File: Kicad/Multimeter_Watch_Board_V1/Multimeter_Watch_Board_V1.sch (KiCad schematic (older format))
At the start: 38 parts, among them J1 AudioJack3_Ground_renamedPins, J2 AudioJack3_Ground_renamedPins, J3 AudioJack3_Ground_renamedPins, J4 Conn_01x16_Female, J5 Conn_01x16_Female, U1 PCF85163-SO08, U2 AD8592, Y1 32kHz

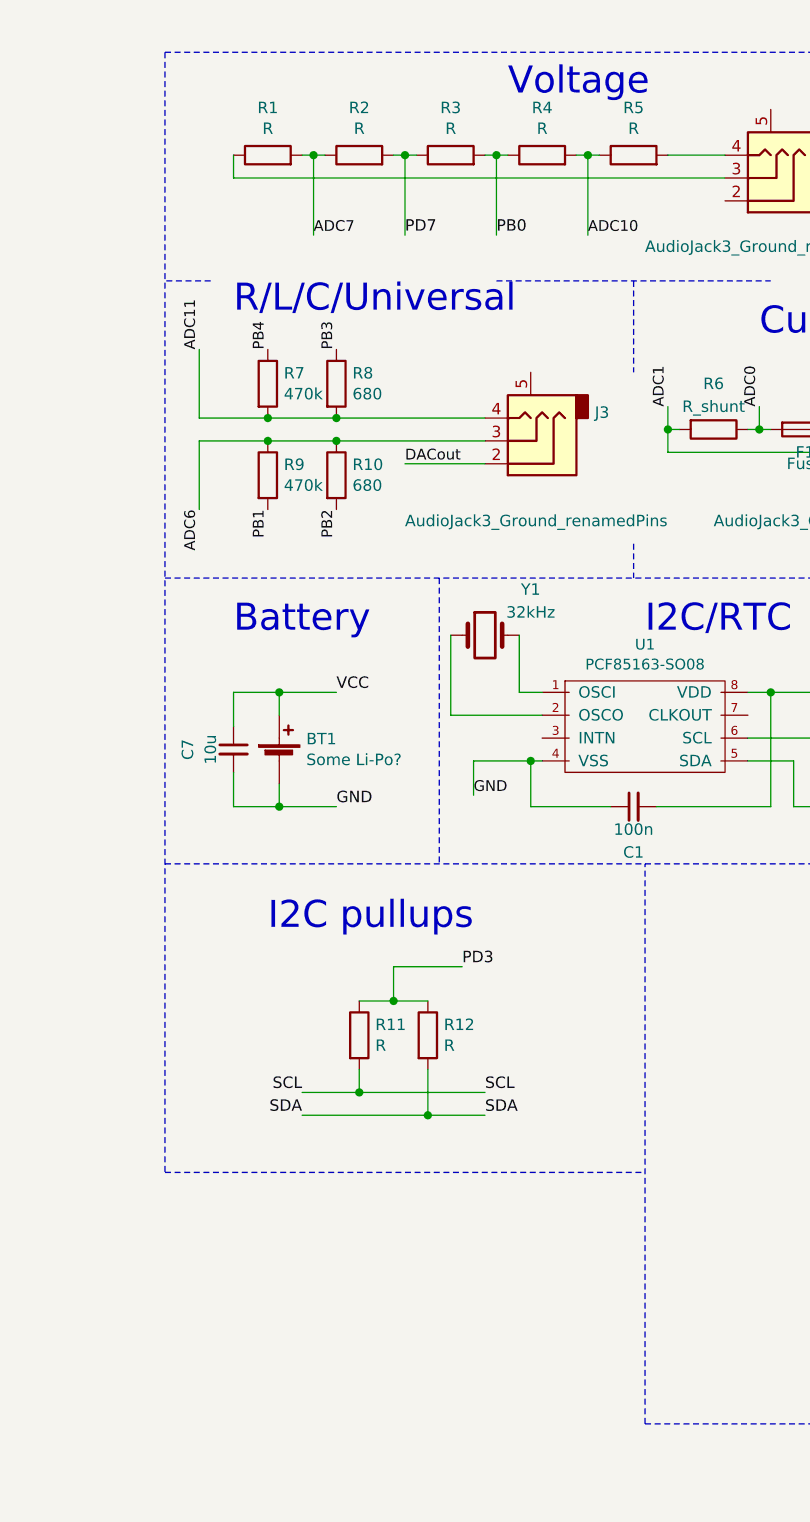
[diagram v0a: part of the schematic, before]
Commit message: reset pullup
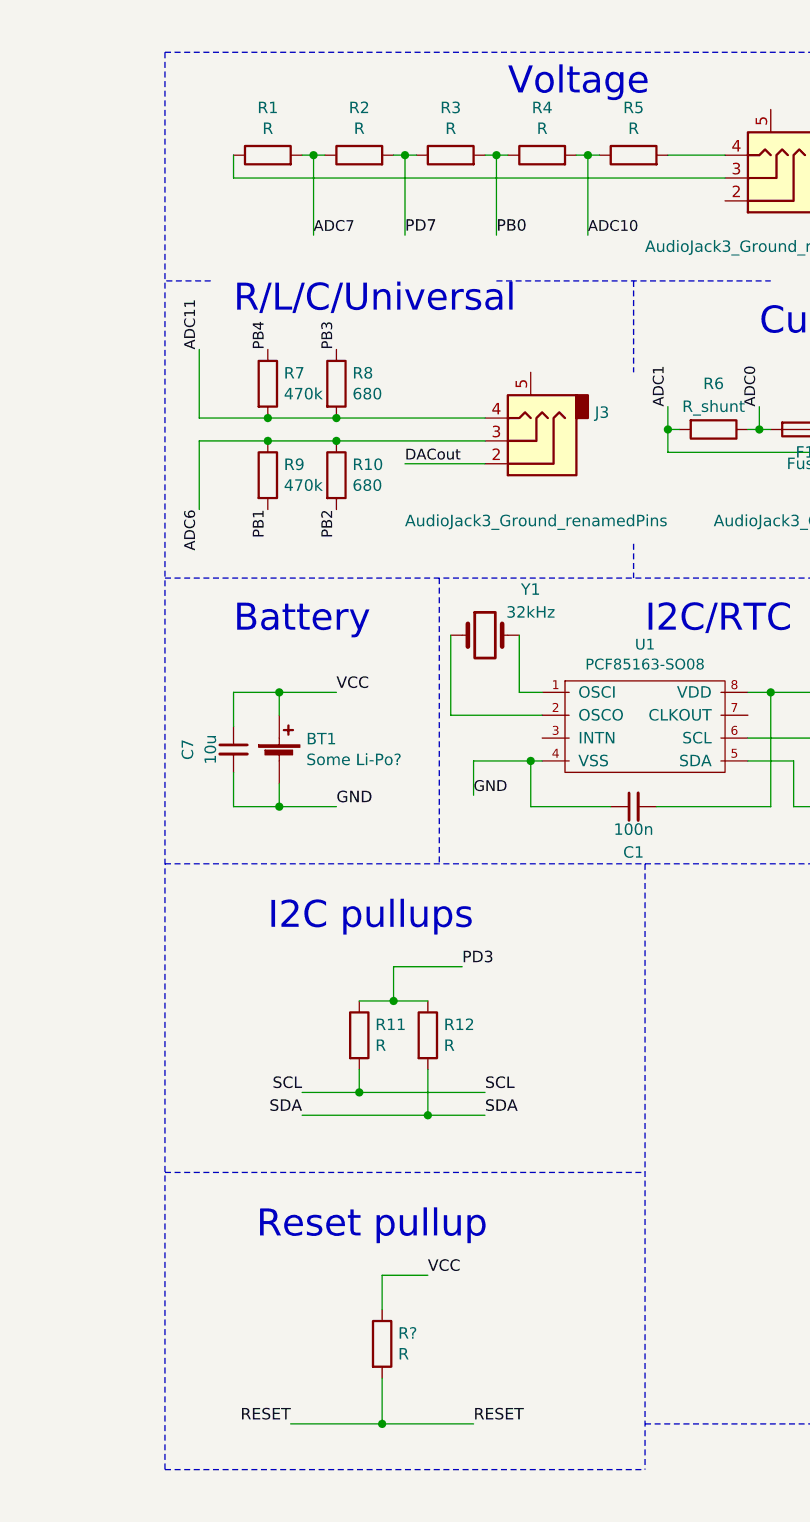
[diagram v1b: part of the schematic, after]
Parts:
- added R?: R, Resistor_SMD:R_0603_1608Metric_Pad1.05x0.95mm_HandSolder, symbol Device:R
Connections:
- net RESET: now also R?.2
- net VCC: now also R?.1
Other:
- note added: "Reset pullup\n"
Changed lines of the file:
@@
 EESchema Schematic File Version 4
-LIBS:Multimeter_Watch_Board_V1-cache
-EELAYER 26 0
+EELAYER 30 0
 EELAYER END
 $Descr A4 11693 8268
@@
 Wire Notes Line
 	11200 500  11200 6500
-Wire Notes Line
-	7000 6500 7000 4050
 $Comp
 L Device:C_Small C2
@@
 Wire Notes Line
 	4900 5400 7000 5400
-Wire Notes Line
-	4900 500  4900 5400
 Wire Wire Line
 	5750 4650 5900 4650
@@
 	-1   0    0    1
 $EndComp
+Text Notes 5300 5700 0    118  ~ 0
+Reset pullup\n
+Text Label 5450 6500 2    50   ~ 0
+RESET
+Text Label 6250 6500 0    50   ~ 0
+RESET
+Wire Wire Line
+	5850 6300 5850 6500
+$Comp
+L Device:R R?
+U 1 1 5F23EEDA
+P 5850 6150
+F 0 "R?" H 5920 6196 50  0000 L CNN
+F 1 "R" H 5920 6105 50  0000 L CNN
+F 2 "Resistor_SMD:R_0603_1608Metric_Pad1.05x0.95mm_HandSolder" V 5780 6150 50  0001 C CNN
+F 3 "~" H 5850 6150 50  0001 C CNN
+	1    5850 6150
+	1    0    0    -1
+$EndComp
+Connection ~ 5850 6500
+Wire Wire Line
+	5850 6500 6250 6500
+Wire Wire Line
+	5450 6500 5850 6500
+Wire Wire Line
+	5850 6000 5850 5850
+Wire Wire Line
+	5850 5850 6050 5850
+Text Label 6050 5850 0    50   ~ 0
+VCC
+Wire Notes Line
+	4900 6700 7000 6700
+Wire Notes Line
+	7000 4050 7000 6700
+Wire Notes Line
+	4900 500  4900 6700
 $EndSCHEMATC
